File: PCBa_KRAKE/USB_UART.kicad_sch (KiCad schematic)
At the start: 21 parts, among them J501 USB_C_Receptacle_USB2.0, Q205 MMBT2222A-7-F, U501 CH340T

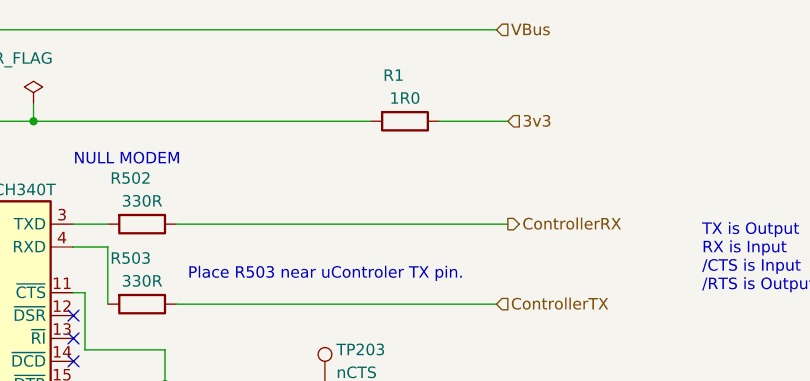
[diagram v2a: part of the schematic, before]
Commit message: Routing and connecting Encoder and 5V.
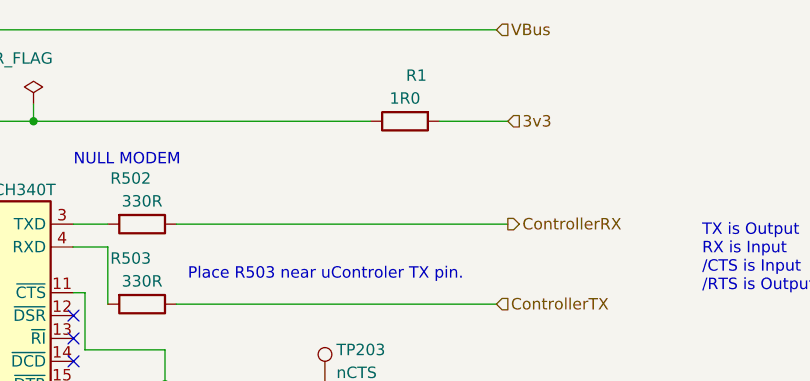
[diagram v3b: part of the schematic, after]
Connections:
- net 3v3: now also R1.2; no longer R1.1
- net at C501.1, C502.1, R1.2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: now also R1.1; no longer R1.2
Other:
- moved on the sheet: R1
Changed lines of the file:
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@@
     )
   )
-  (symbol (lib_id "Device:R") (at 201.93 76.2 270) (unit 1)
+  (symbol (lib_id "Device:R") (at 201.93 76.2 90) (mirror x) (unit 1)
     (in_bom yes) (on_board yes) (dnp no)
-    (property "Reference" "R1" (at 200.66 71.12 90)
+    (property "Reference" "R1" (at 203.2 71.12 90)
       (effects (font (size 1.27 1.27)))
     )

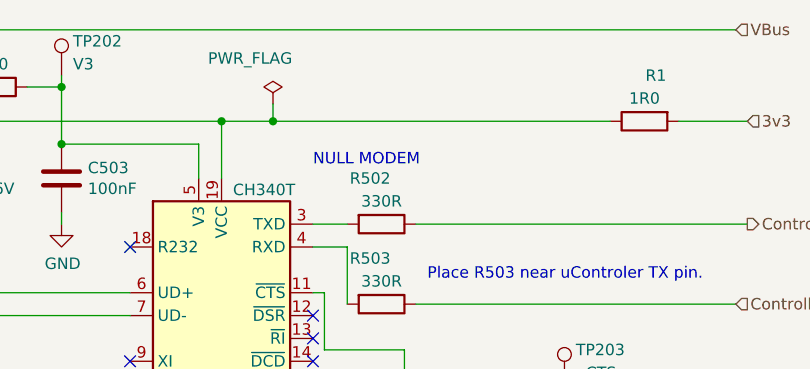
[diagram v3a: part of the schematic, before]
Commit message: Corrected the voltage connection for the mute switch, from 5V to 3V3. Rerouted and reconnected the tracks for R603.
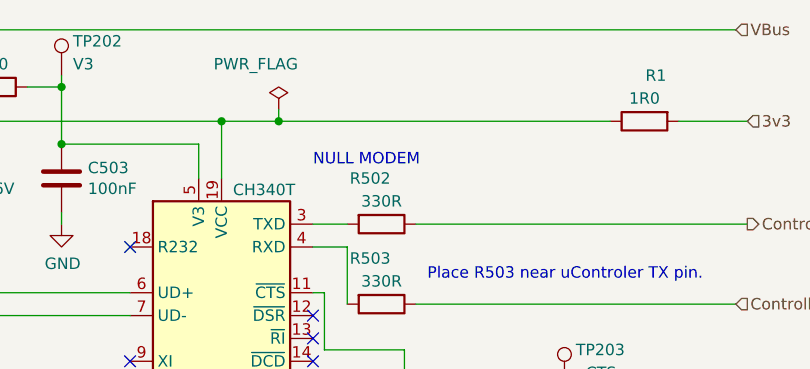
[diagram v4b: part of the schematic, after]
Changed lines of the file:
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@@
   (junction (at 86.36 95.25) (diameter 0) (color 0 0 0 0)
   )
-  (junction (at 160.655 76.2) (diameter 0) (color 0 0 0 0)
+  (junction (at 161.29 76.2) (diameter 0) (color 0 0 0 0)
   )
   (junction (at 175.26 105.41) (diameter 0) (color 0 0 0 0)
@@
     (stroke (width 0) (type default))
   )
-  (wire (pts (xy 160.655 74.295) (xy 160.655 76.2))
+  (wire (pts (xy 161.29 74.93) (xy 161.29 76.2))
     (stroke (width 0) (type default))
   )
@@
     (stroke (width 0) (type default))
   )
-  (wire (pts (xy 160.655 76.2) (xy 198.12 76.2))
+  (wire (pts (xy 161.29 76.2) (xy 198.12 76.2))
     (stroke (width 0) (type default))
   )
@@
     (stroke (width 0) (type default))
   )
-  (wire (pts (xy 154.94 76.2) (xy 160.655 76.2))
+  (wire (pts (xy 154.94 76.2) (xy 161.29 76.2))
     (stroke (width 0) (type default))
   )
@@
     )
   )
-  (symbol (lib_id "power:PWR_FLAG") (at 160.655 74.295 0) (unit 1)
-    (in_bom yes) (on_board yes) (dnp no)
-    (property "Reference" "#FLG0101" (at 160.655 72.39 0)
-      (effects (font (size 1.27 1.27)) hide)
-    )
-    (property "Value" "PWR_FLAG" (at 158.115 69.215 0)
-      (effects (font (size 1.27 1.27)))
-    )
-    (property "Footprint" "" (at 160.655 74.295 0)
-      (effects (font (size 1.27 1.27)) hide)
-    )
-    (property "Datasheet" "~" (at 160.655 74.295 0)
-      (effects (font (size 1.27 1.27)) hide)
-    )
+  (symbol (lib_id "power:PWR_FLAG") (at 161.29 74.93 0) (unit 1)
+    (in_bom yes) (on_board yes) (dnp no)
+    (property "Reference" "#FLG0101" (at 161.29 73.025 0)
+      (effects (font (size 1.27 1.27)) hide)
+    )
+    (property "Value" "PWR_FLAG" (at 158.75 69.85 0)
+      (effects (font (size 1.27 1.27)))
+    )
+    (property "Footprint" "" (at 161.29 74.93 0)
+      (effects (font (size 1.27 1.27)) hide)
+    )
+    (property "Datasheet" "~" (at 161.29 74.93 0)
+      (effects (font (size 1.27 1.27)) hide)
+    )

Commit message: Adding new CH340T footprint. Fixing through hole pads and routings.
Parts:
- U501: footprint Package_SO:SSOP-20_5.3x7.2mm_P0.65mm -> GeneralPurposeAlarmDevicePCB:SSOP-20_5.3x7.2mm_P0.65mm_CH340T
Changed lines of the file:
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@@
       (effects (font (size 1.27 1.27)) (justify left))
     )
-    (property "Footprint" "Package_SO:SSOP-20_5.3x7.2mm_P0.65mm" (at 177.8 125.73 0)
+    (property "Footprint" "GeneralPurposeAlarmDevicePCB:SSOP-20_5.3x7.2mm_P0.65mm_CH340T" (at 177.8 125.73 0)
       (effects (font (size 1.27 1.27)) hide)
     )

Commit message: Found missing part numbers. ESP32.
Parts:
- TP201, TP202: Distributor 1 (none) -> JLCPCB; Distributor 1 PN (none) -> C5277086
- TP203: Distributor 1 (none) -> JLCPCB; Distributor 1 PN (none) -> C5199804
- U501: Distributor 1 (none) -> JLCPCB; Distributor 1 PN (none) -> C8689; MPN (none) -> CH340T; Manufacturer (none) -> WCH(Jiangsu Qin Heng)
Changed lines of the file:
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@@
+      (effects (font (size 1.27 1.27)) hide)
+    )
+    (property "Description" "Test Points/Test Rings ROHS red" (at 102.87 72.39 0)
+      (effects (font (size 1.27 1.27)) hide)
+    )
+    (property "Distributor 1" "JLCPCB" (at 102.87 72.39 0)
+      (effects (font (size 1.27 1.27)) hide)
+    )
+    (property "Distributor 1 PN" "C5277086" (at 102.87 72.39 0)
       (effects (font (size 1.27 1.27)) hide)
     )
@@
       (effects (font (size 1.27 1.27)) hide)
     )
+    (property "Description" "Test Points/Test Rings ROHS red" (at 137.16 71.12 0)
+      (effects (font (size 1.27 1.27)) hide)
+    )
+    (property "Distributor 1" "JLCPCB" (at 137.16 71.12 0)
+      (effects (font (size 1.27 1.27)) hide)
+    )
+    (property "Distributor 1 PN" "C5277086" (at 137.16 71.12 0)
+      (effects (font (size 1.27 1.27)) hide)
+    )
     (pin "1")
     (instances
@@
     )
     (property "Datasheet" "https://cdn.sparkfun.com/datasheets/Dev/Arduino/Other/CH340DS1.PDF" (at 148.59 83.82 0)
+      (effects (font (size 1.27 1.27)) hide)
+    )
+    (property "Distributor 1" "JLCPCB" (at 154.94 105.41 0)
+      (effects (font (size 1.27 1.27)) hide)
+    )
+    (property "Description" "2Mbps Transceiver USB 2.0 SSOP-20-209mil USB Converters ROHS" (at 154.94 105.41 0)
+      (effects (font (size 1.27 1.27)) hide)
+    )
+    (property "Distributor 1 PN" "C8689" (at 154.94 105.41 0)
+      (effects (font (size 1.27 1.27)) hide)
+    )
+    (property "MPN" "CH340T" (at 154.94 105.41 0)
+      (effects (font (size 1.27 1.27)) hide)
+    )
+    (property "Manufacturer" "WCH(Jiangsu Qin Heng)" (at 154.94 105.41 0)
       (effects (font (size 1.27 1.27)) hide)
     )
@@
       (effects (font (size 1.27 1.27)) hide)
     )
+    (property "Distributor 1" "JLCPCB" (at 193.04 105.41 0)
+      (effects (font (size 1.27 1.27)) hide)
+    )
+    (property "Description" "Test Points/Test Rings ROHS yellow" (at 193.04 105.41 0)
+      (effects (font (size 1.27 1.27)) hide)
+    )
+    (property "Distributor 1 PN" "C5199804" (at 193.04 105.41 0)
+      (effects (font (size 1.27 1.27)) hide)
+    )

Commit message: Adding component information. Deleted a redundant LED from the schematic.
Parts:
- J501: MPN (none) -> TYPE-C-31-M-12; Manufacturer (none) -> Korean Hroparts Elec
- TP201, TP202: Cost (none) -> 0.0717; MPN (none) -> RH-5000; Manufacturer (none) -> ronghe
- TP203: Cost (none) -> 0.0800; MPN (none) -> RH-5004; Manufacturer (none) -> ronghe
- U501: AssemblyType (none) -> SMT; Cost (none) -> 0.72
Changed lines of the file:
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@@
+      (effects (font (size 1.27 1.27)) hide)
+    )
+    (property "Description" "47uF 16V 33mA@120Hz ±20% SMD,D5xL5.4mm Aluminum Electrolytic Capacitors - SMD ROHS" (at 120.65 82.55 0)
       (effects (font (size 1.27 1.27)) hide)
     )
@@
       (effects (font (size 1.27 1.27)) hide)
     )
+    (property "MPN" "RH-5000" (at 102.87 72.39 0)
+      (effects (font (size 1.27 1.27)) hide)
+    )
+    (property "Manufacturer" "ronghe" (at 102.87 72.39 0)
+      (effects (font (size 1.27 1.27)) hide)
+    )
+    (property "Cost" "0.0717" (at 102.87 72.39 0)
+      (effects (font (size 1.27 1.27)) hide)
+    )
     (pin "1")
     (instances
@@
       (effects (font (size 1.27 1.27)) hide)
     )
+    (property "MPN" "RH-5000" (at 137.16 71.12 0)
+      (effects (font (size 1.27 1.27)) hide)
+    )
+    (property "Manufacturer" "ronghe" (at 137.16 71.12 0)
+      (effects (font (size 1.27 1.27)) hide)
+    )
+    (property "Cost" "0.0717" (at 137.16 71.12 0)
+      (effects (font (size 1.27 1.27)) hide)
+    )
     (pin "1")
     (instances
@@
     )
     (property "Manufacturer" "WCH(Jiangsu Qin Heng)" (at 154.94 105.41 0)
+      (effects (font (size 1.27 1.27)) hide)
+    )
+    (property "AssemblyType" "SMT" (at 154.94 105.41 0)
+      (effects (font (size 1.27 1.27)) hide)
+    )
+    (property "Cost" "0.72" (at 154.94 105.41 0)
       (effects (font (size 1.27 1.27)) hide)
     )
@@
       (effects (font (size 1.27 1.27)) hide)
     )
+    (property "MPN" "RH-5004" (at 193.04 105.41 0)
+      (effects (font (size 1.27 1.27)) hide)
+    )
+    (property "Manufacturer" "ronghe" (at 193.04 105.41 0)
+      (effects (font (size 1.27 1.27)) hide)
+    )
+    (property "Cost" "0.0800" (at 193.04 105.41 0)
+      (effects (font (size 1.27 1.27)) hide)
+    )
     (pin "1")
     (instances
@@
       (effects (font (size 1.27 1.27)) hide)
     )
+    (property "Description" "5A 1 16P Female Type-C SMD USB Connectors ROHS" (at 71.12 102.87 0)
+      (effects (font (size 1.27 1.27)) hide)
+    )
+    (property "MPN" "TYPE-C-31-M-12" (at 71.12 102.87 0)
+      (effects (font (size 1.27 1.27)) hide)
+    )
+    (property "Manufacturer" "Korean Hroparts Elec" (at 71.12 102.87 0)
+      (effects (font (size 1.27 1.27)) hide)
+    )

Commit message: Editting bulk editor feilds.
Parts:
- J501: AssemblyType (none) -> SMT
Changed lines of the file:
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@@
+      (effects (font (size 1.27 1.27)) hide)
+    )
+    (property "MPN 2" "" (at 172.72 87.63 0)
+      (effects (font (size 1.27 1.27)) hide)
+    )
+    (property "Manufacturer 2" "" (at 172.72 87.63 0)
       (effects (font (size 1.27 1.27)) hide)
     )
@@
     )
     (property "Cost" "0.0015" (at 172.72 96.52 0)
+      (effects (font (size 1.27 1.27)) hide)
+    )
+    (property "MPN 2" "" (at 172.72 96.52 0)
+      (effects (font (size 1.27 1.27)) hide)
+    )
+    (property "Manufacturer 2" "" (at 172.72 96.52 0)
       (effects (font (size 1.27 1.27)) hide)
     )
@@
       (effects (font (size 1.27 1.27)) hide)
     )
+    (property "MPN 2" "" (at 137.16 82.55 0)
+      (effects (font (size 1.27 1.27)) hide)
+    )
+    (property "Manufacturer 2" "" (at 137.16 82.55 0)
+      (effects (font (size 1.27 1.27)) hide)
+    )
     (pin "1")
     (pin "2")
@@
       (effects (font (size 1.27 1.27)) hide)
     )
+    (property "MPN 2" "" (at 120.65 82.55 0)
+      (effects (font (size 1.27 1.27)) hide)
+    )
+    (property "Manufacturer 2" "" (at 120.65 82.55 0)
+      (effects (font (size 1.27 1.27)) hide)
+    )
     (pin "1")
     (pin "2")
@@
       (effects (font (size 1.27 1.27)) hide)
     )
+    (property "MPN 2" "" (at 106.68 82.55 0)
+      (effects (font (size 1.27 1.27)) hide)
+    )
+    (property "Manufacturer 2" "" (at 106.68 82.55 0)
+      (effects (font (size 1.27 1.27)) hide)
+    )
     (pin "1")
     (pin "2")
@@
     )
     (property "Cost" "0.0015" (at 133.35 121.92 0)
+      (effects (font (size 1.27 1.27)) hide)
+    )
+    (property "MPN 2" "" (at 133.35 121.92 0)
+      (effects (font (size 1.27 1.27)) hide)
+    )
+    (property "Manufacturer 2" "" (at 133.35 121.92 0)
       (effects (font (size 1.27 1.27)) hide)
     )
@@
       (effects (font (size 1.27 1.27)) hide)
     )
+    (property "MPN 2" "" (at 121.92 121.92 0)
+      (effects (font (size 1.27 1.27)) hide)
+    )
+    (property "Manufacturer 2" "" (at 121.92 121.92 0)
+      (effects (font (size 1.27 1.27)) hide)
+    )
     (pin "1")
     (pin "2")
@@
       (effects (font (size 1.27 1.27)) hide)
     )
+    (property "MPN 2" "" (at 175.26 110.49 0)
+      (effects (font (size 1.27 1.27)) hide)
+    )
+    (property "Manufacturer 2" "" (at 175.26 110.49 0)
+      (effects (font (size 1.27 1.27)) hide)
+    )
     (pin "1")
     (pin "2")
@@
     )
     (property "Cost" "0.0015" (at 201.93 76.2 0)
+      (effects (font (size 1.27 1.27)) hide)
+    )
+    (property "MPN 2" "" (at 201.93 76.2 0)
+      (effects (font (size 1.27 1.27)) hide)
+    )
+    (property "Manufacturer 2" "" (at 201.93 76.2 0)
       (effects (font (size 1.27 1.27)) hide)
     )
@@
       (effects (font (size 1.27 1.27)) hide)
     )
+    (property "MPN 2" "" (at 102.87 72.39 0)
+      (effects (font (size 1.27 1.27)) hide)
+    )
+    (property "Manufacturer 2" "" (at 102.87 72.39 0)
+      (effects (font (size 1.27 1.27)) hide)
+    )
     (pin "1")
     (instances
@@
     )
     (property "Cost" "0.0015" (at 129.54 72.39 0)
+      (effects (font (size 1.27 1.27)) hide)
+    )
+    (property "MPN 2" "" (at 129.54 72.39 0)
+      (effects (font (size 1.27 1.27)) hide)
+    )
+    (property "Manufacturer 2" "" (at 129.54 72.39 0)
       (effects (font (size 1.27 1.27)) hide)
     )
@@
       (effects (font (size 1.27 1.27)) hide)
     )
+    (property "MPN 2" "" (at 137.16 71.12 0)
+      (effects (font (size 1.27 1.27)) hide)
+    )
+    (property "Manufacturer 2" "" (at 137.16 71.12 0)
+      (effects (font (size 1.27 1.27)) hide)
+    )
     (pin "1")
     (instances
@@
     )
     (property "Cost" "0.0015" (at 199.39 125.73 0)
+      (effects (font (size 1.27 1.27)) hide)
+    )
+    (property "MPN 2" "" (at 199.39 125.73 0)
+      (effects (font (size 1.27 1.27)) hide)
+    )
+    (property "Manufacturer 2" "" (at 199.39 125.73 0)
       (effects (font (size 1.27 1.27)) hide)
     )
@@
       (effects (font (size 1.27 1.27)) hide)
     )
+    (property "MPN 2" "" (at 208.28 125.73 0)
+      (effects (font (size 1.27 1.27)) hide)
+    )
+    (property "Manufacturer 2" "" (at 208.28 125.73 0)
+      (effects (font (size 1.27 1.27)) hide)
+    )
     (pin "1")
     (pin "2")
@@
       (effects (font (size 1.27 1.27)) hide)
     )
+    (property "MPN 2" "" (at 208.28 142.24 0)
+      (effects (font (size 1.27 1.27)) hide)
+    )
+    (property "Manufacturer 2" "" (at 208.28 142.24 0)
+      (effects (font (size 1.27 1.27)) hide)
+    )
     (pin "1")
     (pin "2")
@@
     )
     (property "Cost" "0.72" (at 154.94 105.41 0)
+      (effects (font (size 1.27 1.27)) hide)
+    )
+    (property "MPN 2" "" (at 154.94 105.41 0)
+      (effects (font (size 1.27 1.27)) hide)
+    )
+    (property "Manufacturer 2" "" (at 154.94 105.41 0)
       (effects (font (size 1.27 1.27)) hide)
     )
@@
       (effects (font (size 1.27 1.27)) hide)
     )
+    (property "MPN 2" "" (at 193.04 105.41 0)
+      (effects (font (size 1.27 1.27)) hide)
+    )
+    (property "Manufacturer 2" "" (at 193.04 105.41 0)
+      (effects (font (size 1.27 1.27)) hide)
+    )
     (pin "1")
     (instances
@@
     )
     (property "Cost" "0.0009" (at 100.33 110.49 0)
+      (effects (font (size 1.27 1.27)) hide)
+    )
+    (property "MPN 2" "" (at 100.33 110.49 0)
+      (effects (font (size 1.27 1.27)) hide)
+    )
+    (property "Manufacturer 2" "" (at 100.33 110.49 0)
       (effects (font (size 1.27 1.27)) hide)
     )
@@
     )
     (property "Manufacturer" "Korean Hroparts Elec" (at 71.12 102.87 0)
+      (effects (font (size 1.27 1.27)) hide)
+    )
+    (property "AssemblyType" "SMT" (at 71.12 102.87 0)
+      (effects (font (size 1.27 1.27)) hide)
+    )
+    (property "MPN 2" "" (at 71.12 102.87 0)
+      (effects (font (size 1.27 1.27)) hide)
+    )
+    (property "Manufacturer 2" "" (at 71.12 102.87 0)
       (effects (font (size 1.27 1.27)) hide)
     )
@@
       (effects (font (size 1.27 1.27)) hide)
     )
+    (property "MPN 2" "" (at 92.71 113.03 0)
+      (effects (font (size 1.27 1.27)) hide)
+    )
+    (property "Manufacturer 2" "" (at 92.71 113.03 0)
+      (effects (font (size 1.27 1.27)) hide)
+    )
     (pin "1")
     (pin "2")
@@
       (effects (font (size 1.27 1.27)) hide)
     )
+    (property "MPN 2" "" (at 199.39 142.24 0)
+      (effects (font (size 1.27 1.27)) hide)
+    )
+    (property "Manufacturer 2" "" (at 199.39 142.24 0)
+      (effects (font (size 1.27 1.27)) hide)
+    )
